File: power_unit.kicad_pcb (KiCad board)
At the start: 2 copper layers, 100 x 100 mm, 54 parts, among them J1 ATX-20, U1 LM7805_TO220, U2 LM7905_TO220, X1 Power, X2 Address, X3 Data, X4 Mode, X5 Control, X6 Clock, X7 Power SW, X8 Reset SW, X9 Power LED

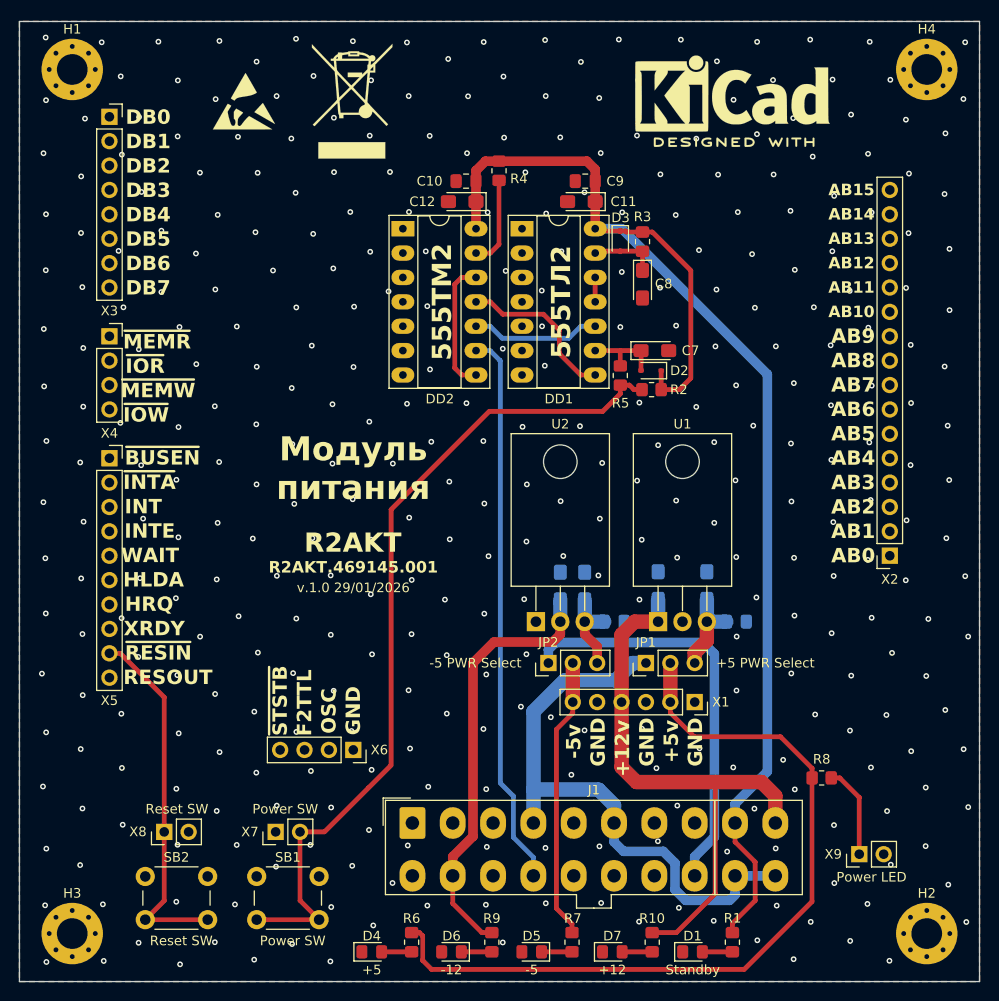
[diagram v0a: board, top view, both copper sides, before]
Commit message: Add files via upload
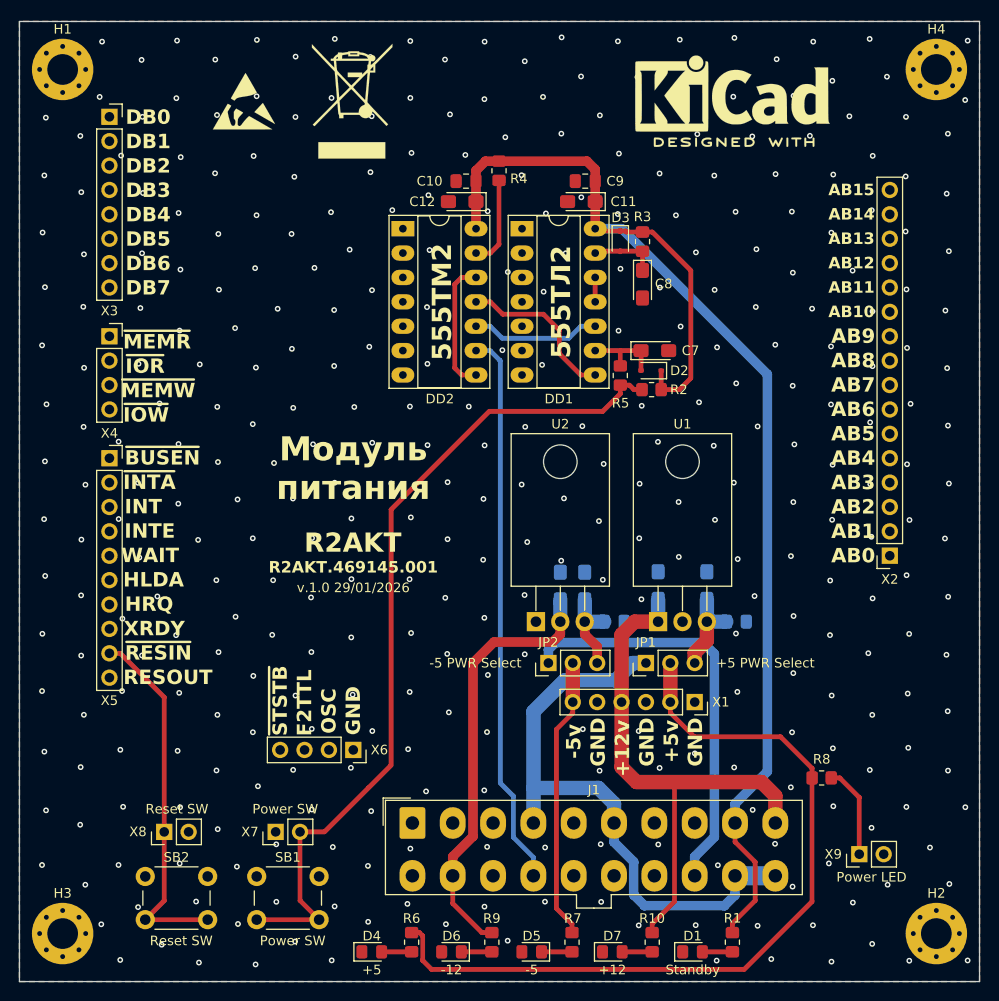
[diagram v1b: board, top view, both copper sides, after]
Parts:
- moved H1 1.00 mm to (66.7, 63.7)
- moved H2 1.00 mm to (157.7, 153.7)
- moved H3 1.00 mm to (66.7, 153.7)
- moved H4 1.00 mm to (157.7, 63.7)
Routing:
- net +12: track 60.4 -> 57.2 mm
- net Net-(JP1-A): track 61.5 -> 62.5 mm
- net GND: vias 367 -> 361

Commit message: Add files via upload
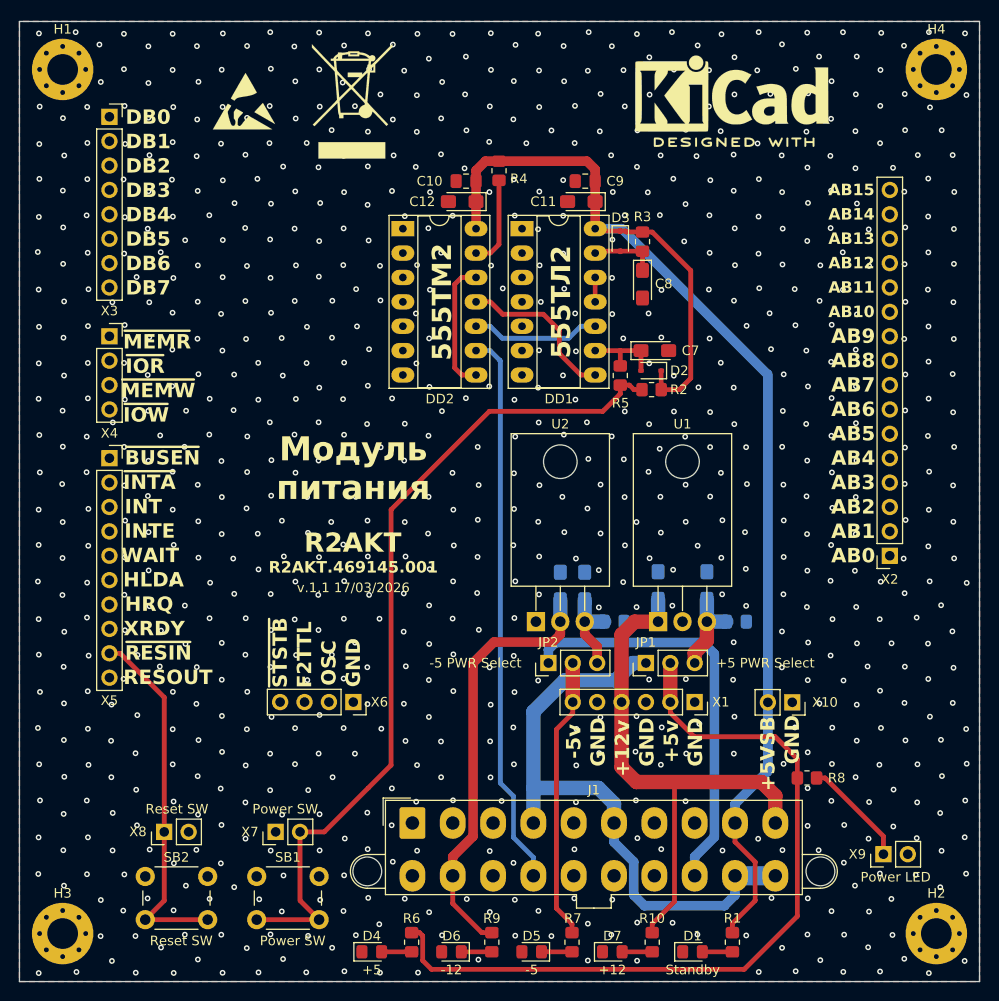
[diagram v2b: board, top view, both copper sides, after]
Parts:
- added X10: RTC Standby, Connector_PinSocket_2.54mm:PinSocket_1x02_P2.54mm_Vertical, F.Cu at (142.7, 129.6)
- J1: footprint Connector_Molex:Molex_Mini-Fit_Jr_5566-20A_2x10_P4.20mm_Vertical -> Connector_Molex:Molex_Mini-Fit_Jr_5566-20A2_2x10_P4.20mm_Vertical
- moved X6 4.98 mm to (97.0, 129.6)
- moved X9 2.51 mm to (152.2, 145.5)
- moved R8 1.53 mm to (144.2, 137.5)
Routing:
- net Net-(X9-Pin_1): track 9.67 -> 11.4 mm
- net +5: track 83.9 -> 82.4 mm
- net GND: vias 361 -> 852
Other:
- board text added: "+5VSB"
- board text added: "v.1.1 17/03/2026"
- board text removed: "v.1.0 29/01/2026"
